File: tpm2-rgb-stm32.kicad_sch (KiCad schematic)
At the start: 59 parts, among them J1 Conn_01x04_Male, J2 Screw_Terminal_01x04, J3 Screw_Terminal_01x02, J4 Screw_Terminal_01x02, J5 12401832E402A, J6 Screw_Terminal_01x04, SW1 SW_Push, U1 COS4426SR, U10 IRF7458TRPBF, U11 IRF7458TRPBF, U12 COS4426SR, U13 IRF7458TRPBF, U14 IRF7458TRPBF, U15 FT232RL, U2 IRF7458TRPBF, U3 IRF7458TRPBF, U4 STM32F103CBTx, U5 COS4426SR, U6 IRF7458TRPBF, U7 IRF7458TRPBF, U8 COS4426SR, U9 LM1117-3.3, Y1 8MHz

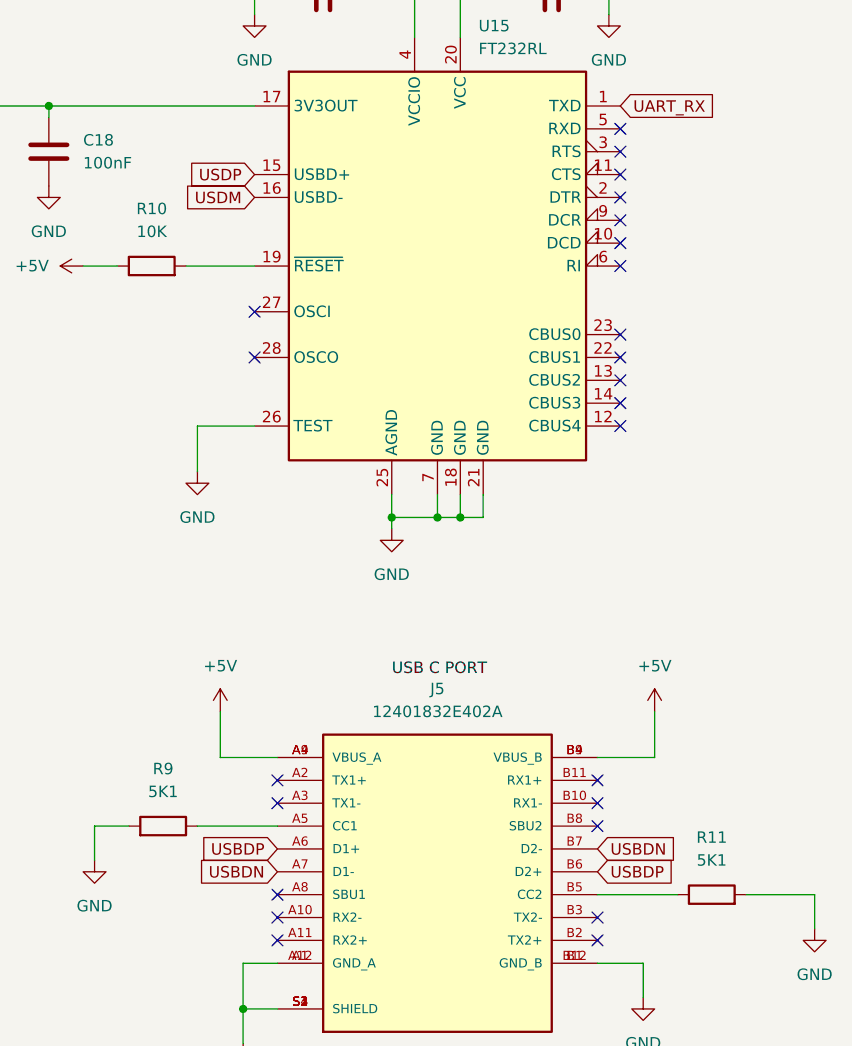
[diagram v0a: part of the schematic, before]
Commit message: Do more routing
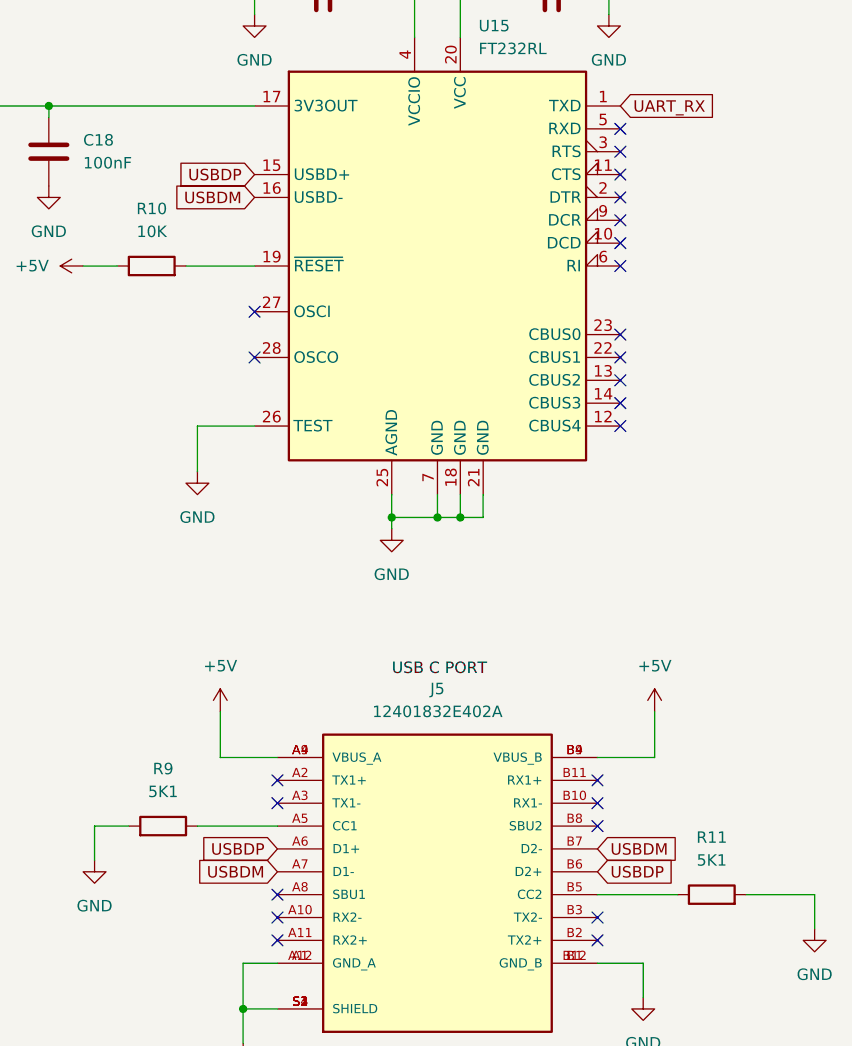
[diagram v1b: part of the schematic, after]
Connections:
- net USDM is gone; now on net USBDM: U15.16 (USBD-)
- net USDP is gone; now on net USBDP: U15.15 (USBD+)
- net USBDN renamed USBDM
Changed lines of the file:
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@@
     )
   )
-  (global_label "USBDN" (shape input) (at 336.55 132.08 0) (fields_autoplaced)
-    (effects (font (size 1.27 1.27)) (justify left))
-    (property "Intersheet References" "${INTERSHEET_REFS}" (id 0) (at 345.3736 132.0006 0)
+  (global_label "USBDM" (shape input) (at 336.55 132.08 0) (fields_autoplaced)
+    (effects (font (size 1.27 1.27)) (justify left))
+    (property "Intersheet References" "${INTERSHEET_REFS}" (id 0) (at 345.4945 132.0006 0)
       (effects (font (size 1.27 1.27)) (justify left) hide)
     )
@@
     )
   )
-  (global_label "USDP" (shape input) (at 298.45 57.15 180) (fields_autoplaced)
-    (effects (font (size 1.27 1.27)) (justify right))
-    (property "Intersheet References" "${INTERSHEET_REFS}" (id 0) (at 290.9569 57.0706 0)
+  (global_label "USBDP" (shape input) (at 298.45 57.15 180) (fields_autoplaced)
+    (effects (font (size 1.27 1.27)) (justify right))
+    (property "Intersheet References" "${INTERSHEET_REFS}" (id 0) (at 289.6869 57.0706 0)
       (effects (font (size 1.27 1.27)) (justify right) hide)
     )
@@
     )
   )
-  (global_label "USBDN" (shape input) (at 300.99 134.62 180) (fields_autoplaced)
-    (effects (font (size 1.27 1.27)) (justify right))
-    (property "Intersheet References" "${INTERSHEET_REFS}" (id 0) (at 292.1664 134.5406 0)
+  (global_label "USBDM" (shape input) (at 300.99 134.62 180) (fields_autoplaced)
+    (effects (font (size 1.27 1.27)) (justify right))
+    (property "Intersheet References" "${INTERSHEET_REFS}" (id 0) (at 292.0455 134.5406 0)
       (effects (font (size 1.27 1.27)) (justify right) hide)
     )
@@
     )
   )
-  (global_label "USDM" (shape input) (at 298.45 59.69 180) (fields_autoplaced)
-    (effects (font (size 1.27 1.27)) (justify right))
-    (property "Intersheet References" "${INTERSHEET_REFS}" (id 0) (at 290.7755 59.6106 0)
-      (effects (font (size 1.27 1.27)) (justify right) hide)
-    )
+  (global_label "USBDM" (shape input) (at 298.45 59.69 180) (fields_autoplaced)
+    (effects (font (size 1.27 1.27)) (justify right))
+    (property "Intersheet References" "${INTERSHEET_REFS}" (id 0) (at 289.5055 59.6106 0)
+      (effects (font (size 1.27 1.27)) (justify right) hide)
+    )
